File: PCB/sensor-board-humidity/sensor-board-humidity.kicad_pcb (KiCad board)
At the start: 2 copper layers, 23.6 x 23.5 mm, 10 parts, among them U1 MAGNETIC POGO CONN., U2 MAGNETIC POGO CONN.

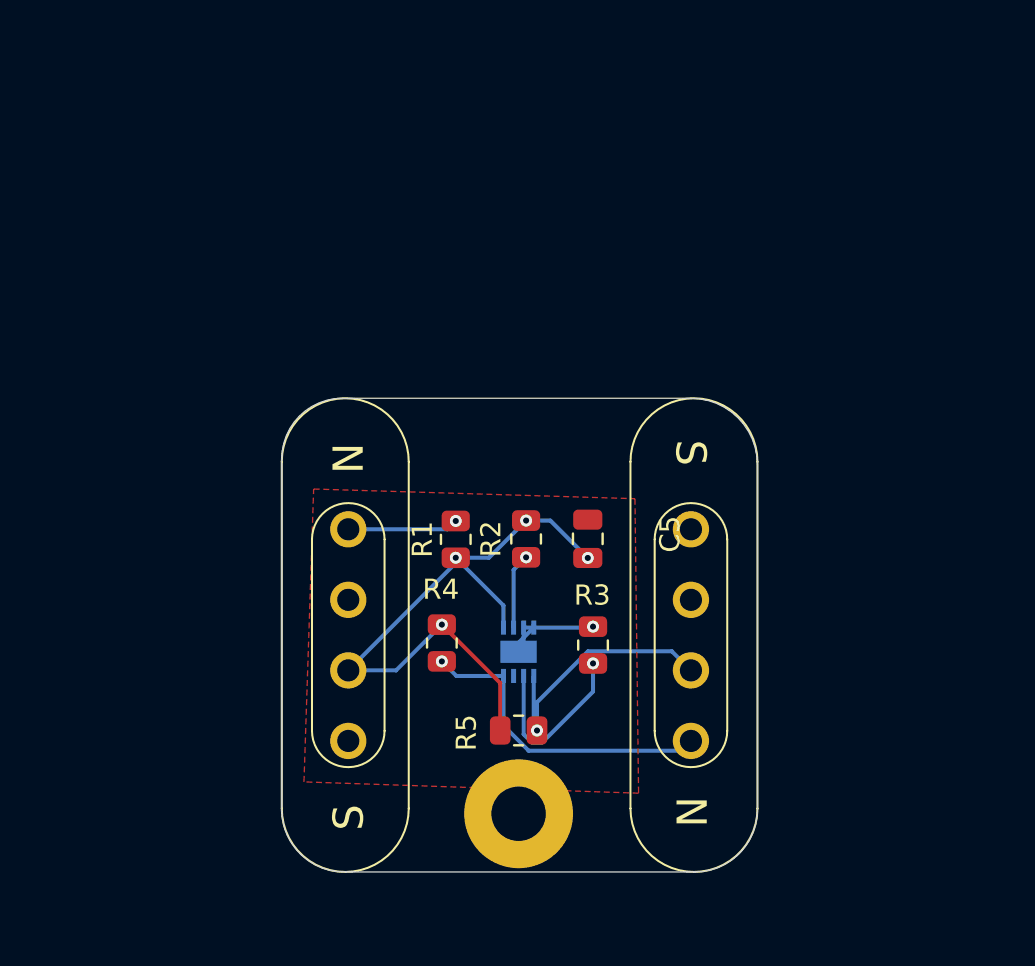
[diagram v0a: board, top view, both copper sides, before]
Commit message: made some changes
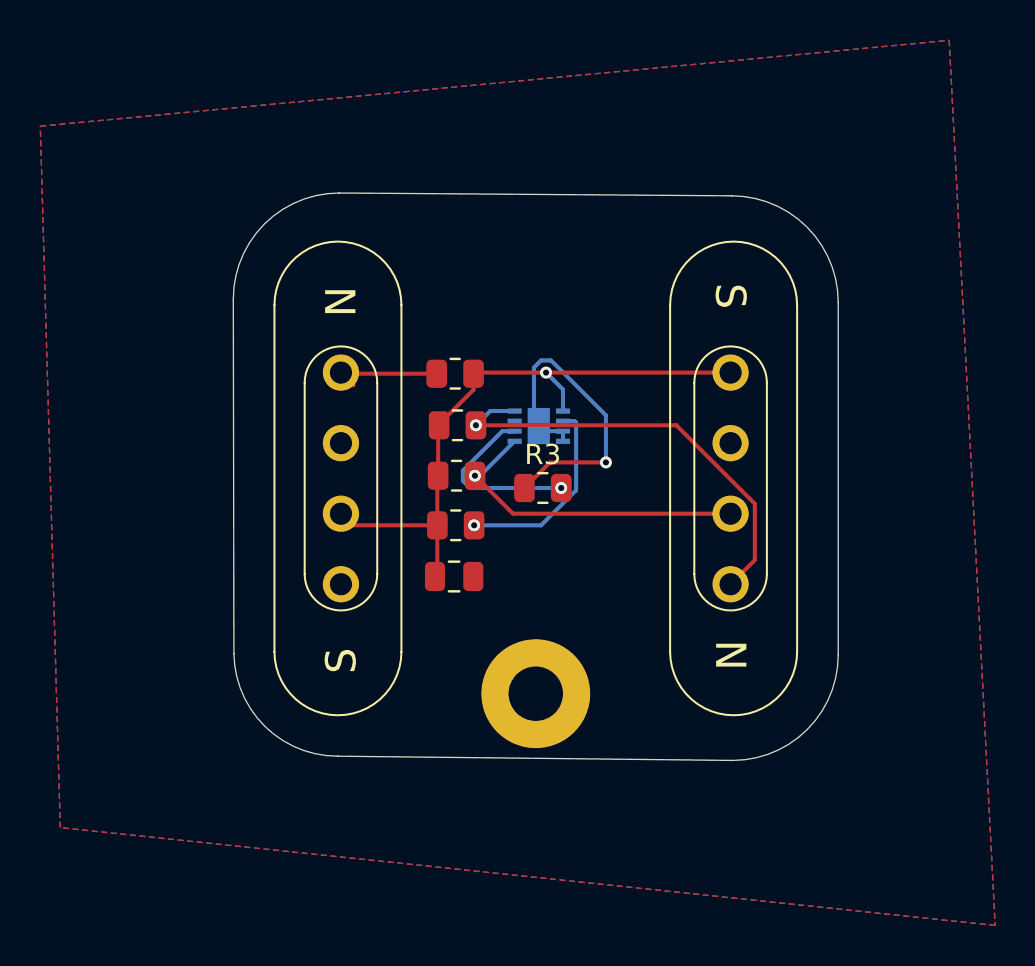
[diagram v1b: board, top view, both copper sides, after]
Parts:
- added G***: LOGO, LOGO, B.Cu at (120.0, 68.7)
- moved R5 13.0 mm to (116.1, 64.2)
- moved SHT31 11.2 mm to (120.2, 61.8), turned to 90 degrees
- moved R4 10.8 mm to (116.1, 61.7), turned to 0 degrees
- moved R1 8.22 mm to (116.0, 59.2), turned to 180 degrees
- moved R3 8.18 mm to (120.4, 64.8), turned to 0 degrees
- moved U1 8.02 mm to (129.7, 64.4)
- moved U2 7.78 mm to (110.4, 64.4)
- moved C5 6.89 mm to (116.0, 69.2), turned to 0 degrees
- moved H1 6.02 mm to (120.0, 75.0)
- moved R2 3.56 mm to (116.1, 66.7), turned to 180 degrees
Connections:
- U1 pad 1: unconnected-(U1-Pad1) -> +3.3V
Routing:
- net GND: track 6.47 -> 16.6 mm
- net /SCL: track 15.8 -> 22.2 mm
- net Net-(SHT31-nRESET): track 3.74 -> 9.82 mm
- net /SDA: track 13.2 -> 16.1 mm
- net +3.3V: track 32.4 -> 30.9 mm, vias 4 -> 1
- net /ID: track 5.50 -> 5.67 mm, vias 1 -> 0
- added copper zone on B.Cu, net GND
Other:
- board size 23.6 x 23.5 mm -> 30 x 28.1 mm
- board text added: "BOREALIS"
- board text added: "Humidity Sensor"
- board text removed: "Borealis Humidity Sensor"
